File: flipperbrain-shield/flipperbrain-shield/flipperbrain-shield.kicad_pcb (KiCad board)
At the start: 2 copper layers, 68.6 x 53.3 mm, 27 parts, among them J1 Power, J2 Digital/PWM, J3 Analog, J4 Digital/PWM, J5 Screw_Terminal_01x06, J6 Screw_Terminal_01x06, SW10 SW_Push, SW11 SW_Push, SW12 SW_Push, SW13 SW_Push, SW8 SW_Push, SW9 SW_Push

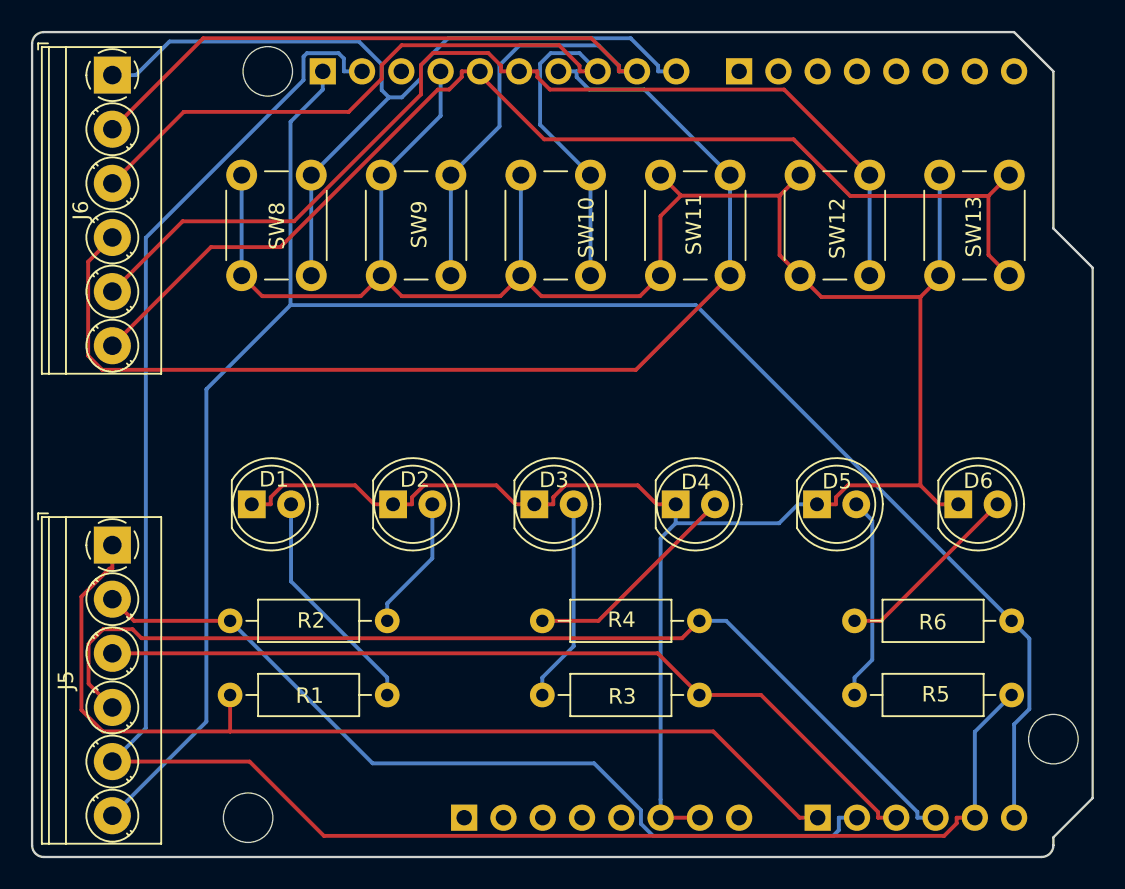
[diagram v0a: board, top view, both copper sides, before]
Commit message: nc
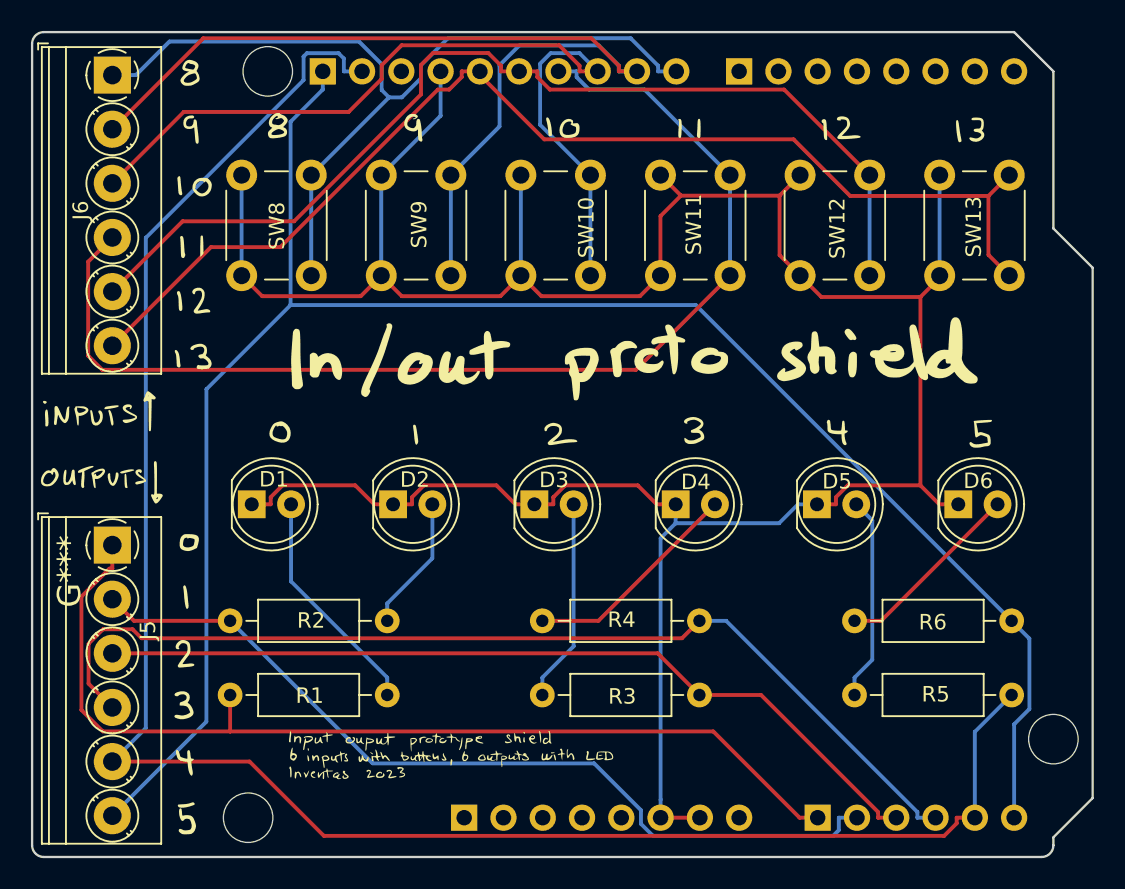
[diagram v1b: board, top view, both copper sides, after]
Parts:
- added G***: LOGO, LOGO, F.Cu at (130.5, 73.7)
